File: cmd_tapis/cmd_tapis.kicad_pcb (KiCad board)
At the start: 2 copper layers, 50 x 40 mm, 12 parts, among them J1 Cmd_12V, J2 IN_230V, J3 OUT_230V, X1 Trou, X2 Trou, X3 Trou, X4 Trou

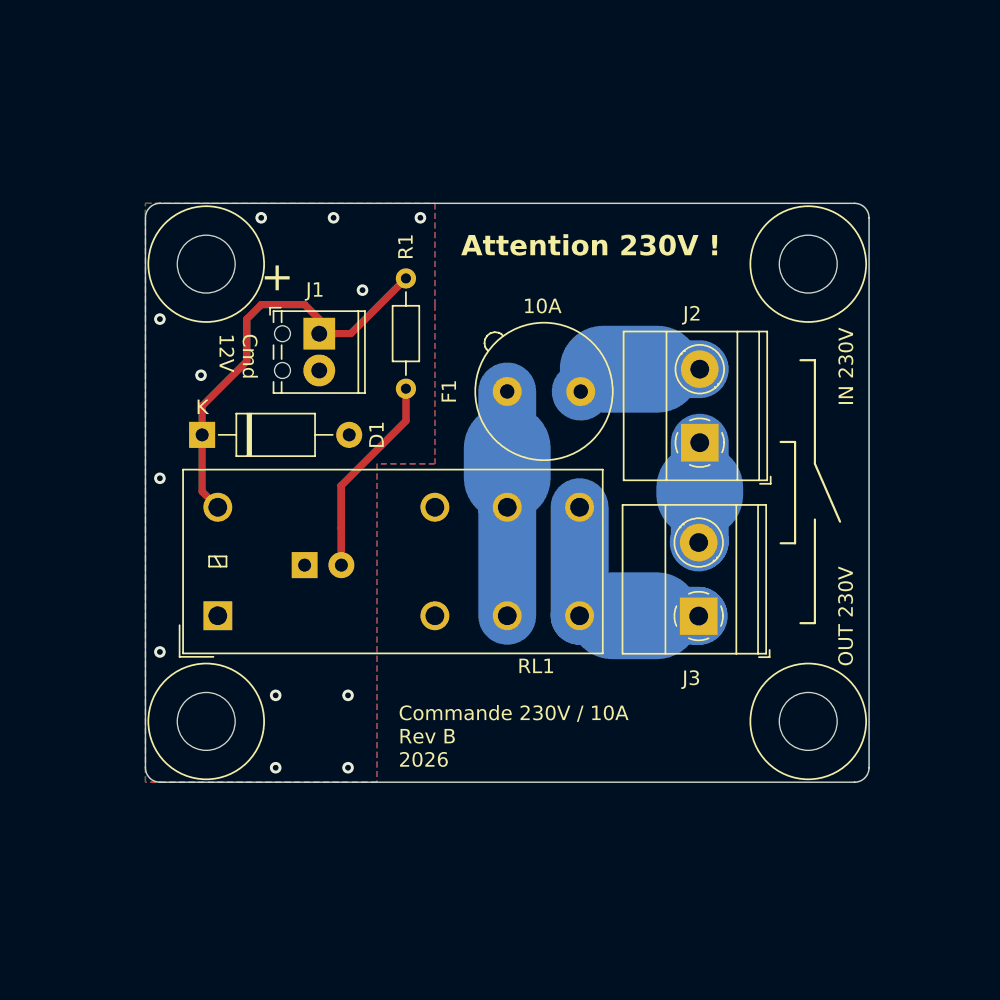
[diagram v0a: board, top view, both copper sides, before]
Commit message: Carte au format de la boite de dérivation
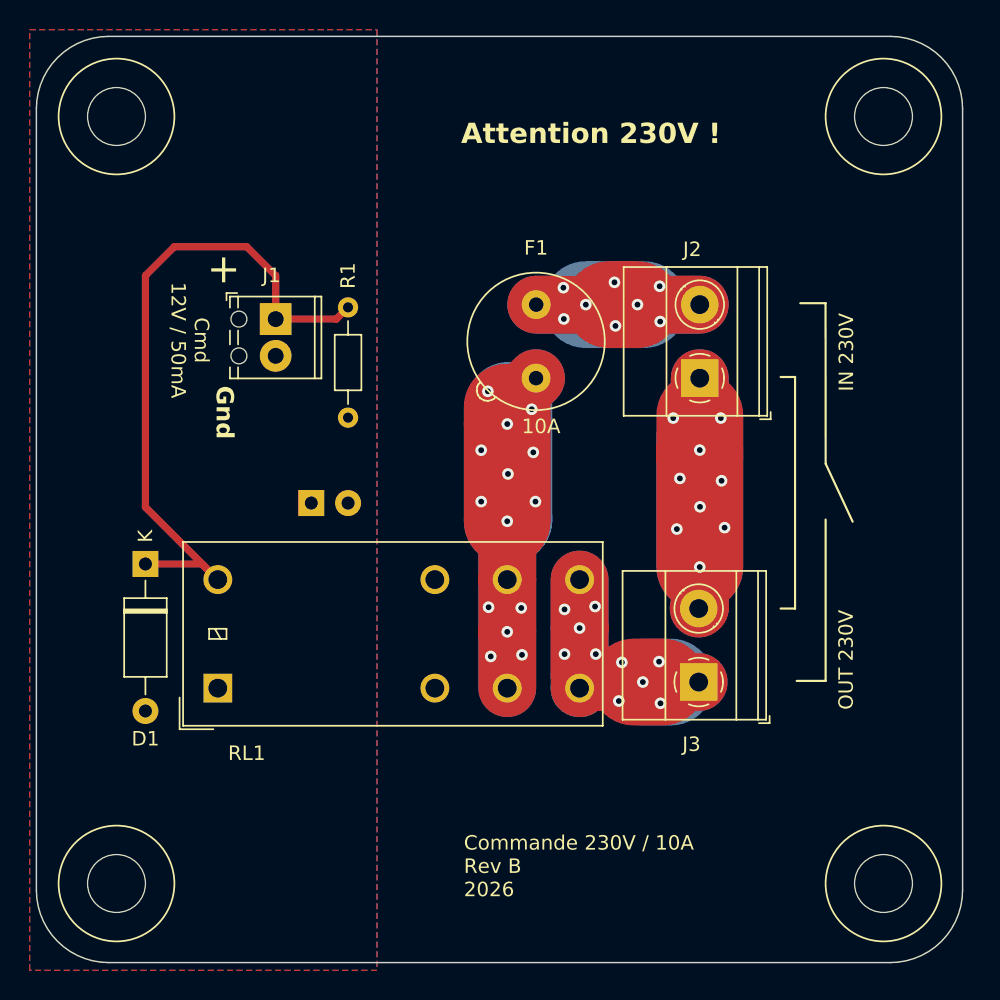
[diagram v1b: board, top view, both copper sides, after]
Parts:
- moved X3 12.8 mm to (128.0, 95.0)
- moved X4 12.3 mm to (181.0, 95.0)
- moved X1 11.9 mm to (128.0, 42.0)
- moved X2 11.4 mm to (181.0, 42.0)
- moved D1 9.74 mm to (130.0, 72.9), turned to -90 degrees
- moved F1 6.75 mm to (157.0, 55.0), turned to -90 degrees
- moved RL1 5.00 mm to (135.0, 81.5)
- moved J3 4.56 mm to (168.2, 81.1)
- moved R1 4.47 mm to (144.0, 55.2)
- moved J2 4.46 mm to (168.3, 60.1)
- moved D2 4.31 mm to (141.5, 68.7)
- moved J1 3.17 mm to (139.0, 56.0)
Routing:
- net Net-(J2-Pin_1): track 7.40 -> 40.9 mm, vias 0 -> 9
- net Net-(F1-Pad2): track 17.6 -> 44.5 mm, vias 0 -> 14
- net Net-(J3-Pin_1): track 15.7 -> 35.5 mm, vias 0 -> 10
- net Net-(D2-A): track 19.6 -> 0.00 mm
- net Net-(D1-K): track 29.1 -> 47.5 mm
- net Net-(J2-Pin_2): track 12.6 -> 22.6 mm, vias 0 -> 8
- net GND: vias 12 -> 0
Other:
- board size 50 x 40 mm -> 64 x 64 mm
- board text added: "Cmd 12V / 50mA"
- board text added: "Gnd"
- board text added: "ON"
- board text removed: "Cmd 12V"

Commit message: Améliorations:
- Isolation renforcée en coupant le PCB
- Ajout de passage pour colliers de serrage des cables
- Ajout diode en direct
- Ajout découplages
- Alignement grille 1mm
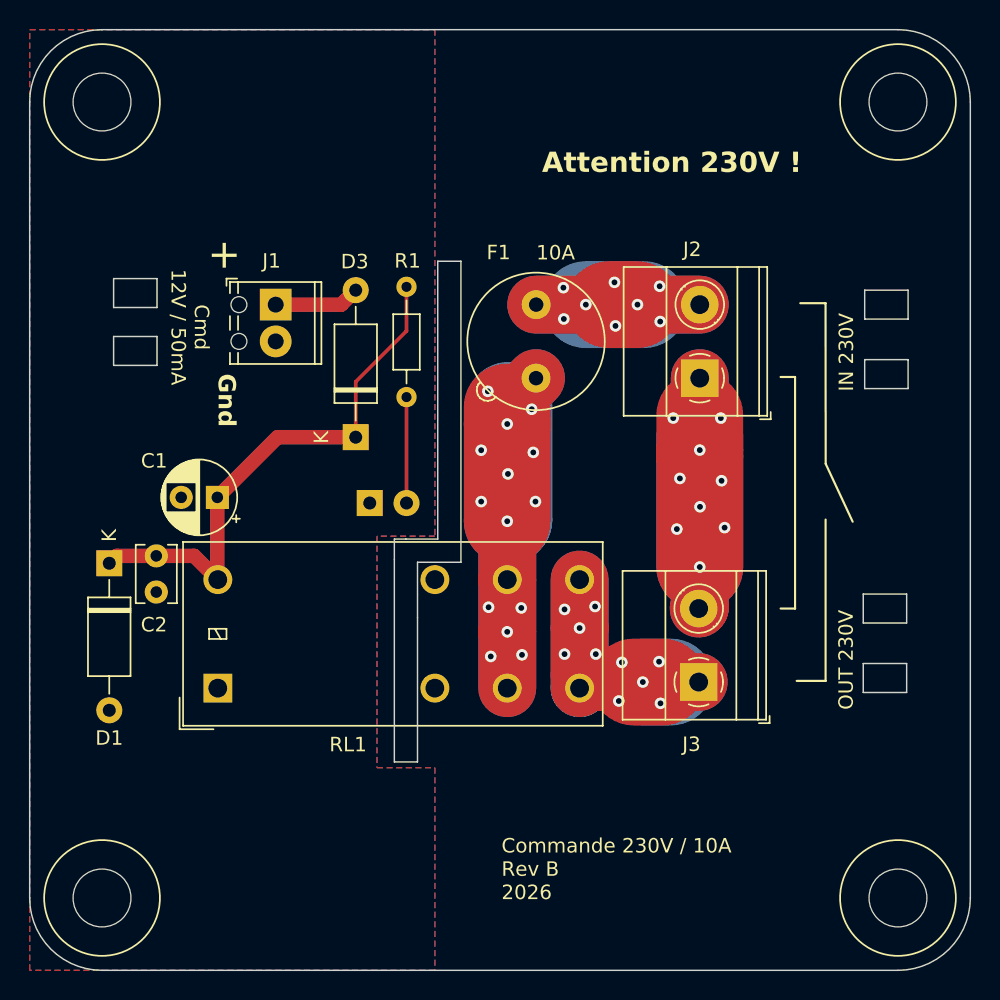
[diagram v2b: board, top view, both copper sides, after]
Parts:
- added C1: 20µF, Capacitor_THT:CP_Radial_D5.0mm_P2.50mm, F.Cu at (135.0, 68.3)
- added C2: 100nF, Capacitor_THT:C_Disc_D3.8mm_W2.6mm_P2.50mm, F.Cu at (130.8, 72.4)
- added D3: 1N5818, Diode_THT:D_A-405_P10.16mm_Horizontal, F.Cu at (144.5, 64.2)
- R1: value R -> 1k
- moved R1 4.28 mm to (148.0, 53.8)
- moved D2 4.04 mm to (145.5, 68.7)
- moved D1 2.50 mm to (127.5, 72.9)
- moved X1 1.41 mm to (127.0, 41.0)
- moved X2 1.41 mm to (182.0, 41.0)
- moved X3 1.41 mm to (127.0, 96.0)
- moved X4 1.41 mm to (182.0, 96.0)
- moved J1 1.00 mm to (139.0, 55.0)
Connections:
- J1 pad 1: Net-(D1-K) -> Net-(D3-A)
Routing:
- net Net-(D1-K): track 47.5 -> 37.2 mm
- net Net-(D2-A): track 0.00 -> 7.32 mm
- net Net-(D3-A): track 0.00 -> 5.94 mm
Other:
- board size 64 x 64 mm -> 65 x 65 mm

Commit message: Retouche dimension PCB 64mm x 64mm
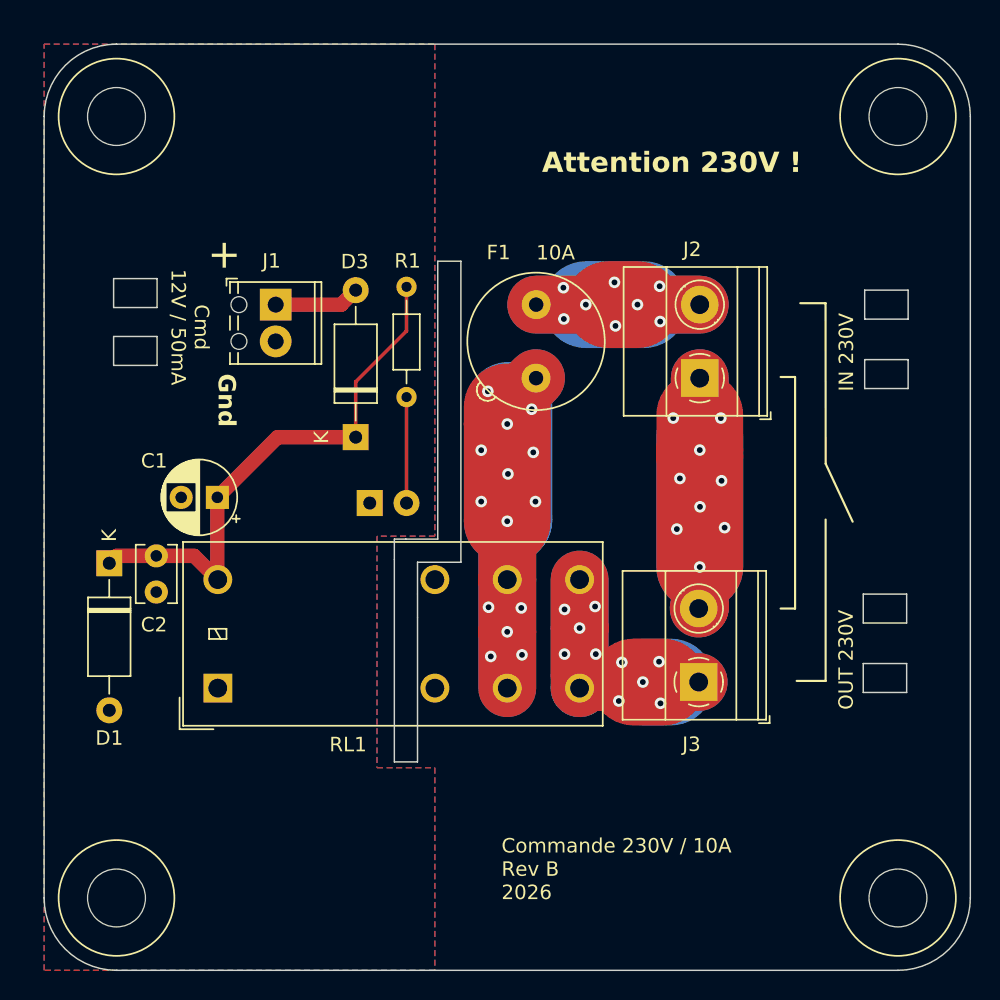
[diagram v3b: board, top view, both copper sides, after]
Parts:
- moved X1 1.41 mm to (128.0, 42.0)
- moved X2 1.00 mm to (182.0, 42.0)
- moved X3 1.00 mm to (128.0, 96.0)
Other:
- board size 65 x 65 mm -> 64 x 64 mm
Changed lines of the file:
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@@
   )
   (footprint "bpc:BPC_Trou4mm_Fixation" (layer "F.Cu")
-    (at 127 96)
+    (at 128 96)
     (property "Sheetfile" "cmd_tapis.kicad_sch")
     (property "Sheetname" "")
@@
   )
   (footprint "bpc:BPC_Trou4mm_Fixation" (layer "F.Cu")
-    (at 182 41)
+    (at 182 42)
     (property "Sheetfile" "cmd_tapis.kicad_sch")
     (property "Sheetname" "")
@@
   )
   (footprint "bpc:BPC_Trou4mm_Fixation" (layer "F.Cu")
-    (at 127 41)
+    (at 128 42)
     (property "Sheetfile" "cmd_tapis.kicad_sch")
     (property "Sheetname" "")
@@
   (gr_arc (start 187 96) (mid 185.535534 99.535534) (end 182 101)
     (stroke (width 0.1) (type default)) (layer "Edge.Cuts"))
+  (gr_arc (start 182 37) (mid 185.535534 38.464466) (end 187 42)
+    (stroke (width 0.1) (type default)) (layer "Edge.Cuts"))
   (gr_line (start 148.8 72.8) (end 148.8 75)
     (stroke (width 0.1) (type default)) (layer "Edge.Cuts"))
   (gr_rect (start 179.7 58.8) (end 182.7 60.8)
     (stroke (width 0.1) (type default)) (fill none) (layer "Edge.Cuts"))
-  (gr_arc (start 122 41) (mid 123.464466 37.464466) (end 127 36)
-    (stroke (width 0.1) (type default)) (layer "Edge.Cuts"))
   (gr_line (start 147.2 72.6) (end 147.2 71.2)
     (stroke (width 0.1) (type default)) (layer "Edge.Cuts"))
   (gr_line (start 147.2 71.2) (end 148 71.2)
     (stroke (width 0.1) (type default)) (layer "Edge.Cuts"))
+  (gr_arc (start 123 42) (mid 124.464466 38.464466) (end 128 37)
+    (stroke (width 0.1) (type default)) (layer "Edge.Cuts"))
   (gr_line (start 150.2 52) (end 150.2 71.2)
-    (stroke (width 0.1) (type default)) (layer "Edge.Cuts"))
-  (gr_arc (start 182 36) (mid 185.535534 37.464466) (end 187 41)
     (stroke (width 0.1) (type default)) (layer "Edge.Cuts"))
   (gr_rect (start 179.6 75) (end 182.6 77)
     (stroke (width 0.1) (type default)) (fill none) (layer "Edge.Cuts"))
-  (gr_line (start 127 36) (end 182 36)
+  (gr_line (start 128 37) (end 182 37)
     (stroke (width 0.1) (type default)) (layer "Edge.Cuts"))
   (gr_line (start 147.2 86.6) (end 147.2 72.6)
     (stroke (width 0.1) (type default)) (layer "Edge.Cuts"))
-  (gr_line (start 187 41) (end 187 96)
-    (stroke (width 0.1) (type default)) (layer "Edge.Cuts"))
-  (gr_line (start 127 101) (end 182 101)
+  (gr_line (start 187 42) (end 187 96)
+    (stroke (width 0.1) (type default)) (layer "Edge.Cuts"))
+  (gr_arc (start 128 101) (mid 124.464466 99.535534) (end 123 96)
+    (stroke (width 0.1) (type default)) (layer "Edge.Cuts"))
+  (gr_line (start 128 101) (end 182 101)
     (stroke (width 0.1) (type default)) (layer "Edge.Cuts"))
   (gr_rect (start 127.8 53.2) (end 130.8 55.2)
@@
   (gr_line (start 151.8 52) (end 151.8 72.8)
     (stroke (width 0.1) (type default)) (layer "Edge.Cuts"))
-  (gr_arc (start 127 101) (mid 123.464466 99.535534) (end 122 96)
-    (stroke (width 0.1) (type default)) (layer "Edge.Cuts"))
   (gr_line (start 150.2 71.2) (end 148 71.2)
     (stroke (width 0.1) (type default)) (layer "Edge.Cuts"))
-  (gr_line (start 122 96) (end 122 41)
+  (gr_line (start 123 96) (end 123 42)
     (stroke (width 0.1) (type default)) (layer "Edge.Cuts"))
   (gr_line (start 151.8 72.8) (end 148.8 72.8)
@@
   )
   (dimension (type aligned) (layer "User.1")
-    (pts (xy 122 36) (xy 122 101))
+    (pts (xy 122 37) (xy 122 101))
     (height 7)
-    (gr_text "65,0000 mm" (at 113.85 68.5 90) (layer "User.1")
+    (gr_text "64,0000 mm" (at 113.85 68.5 90) (layer "User.1")
       (effects (font (size 1 1) (thickness 0.15)))
     )
@@
   )
   (dimension (type aligned) (layer "User.1")
-    (pts (xy 122 36) (xy 187 36))
+    (pts (xy 123 36) (xy 187 36))
     (height -11)
-    (gr_text "65,0000 mm" (at 154.5 23.85) (layer "User.1")
+    (gr_text "64,0000 mm" (at 155 23.85) (layer "User.1")
       (effects (font (size 1 1) (thickness 0.15)))
     )
@@
     (polygon
       (pts
-        (xy 122 36)
-        (xy 150 36)
+        (xy 123 37)
+        (xy 150 37)
         (xy 150 71)
         (xy 146 71)
@@
         (xy 150 87)
         (xy 150 101)
-        (xy 122 101)
+        (xy 123 101)
       )
     )
